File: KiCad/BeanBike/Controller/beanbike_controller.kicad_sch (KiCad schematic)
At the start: 1 part, among them U1 ESP32-WROOM-32

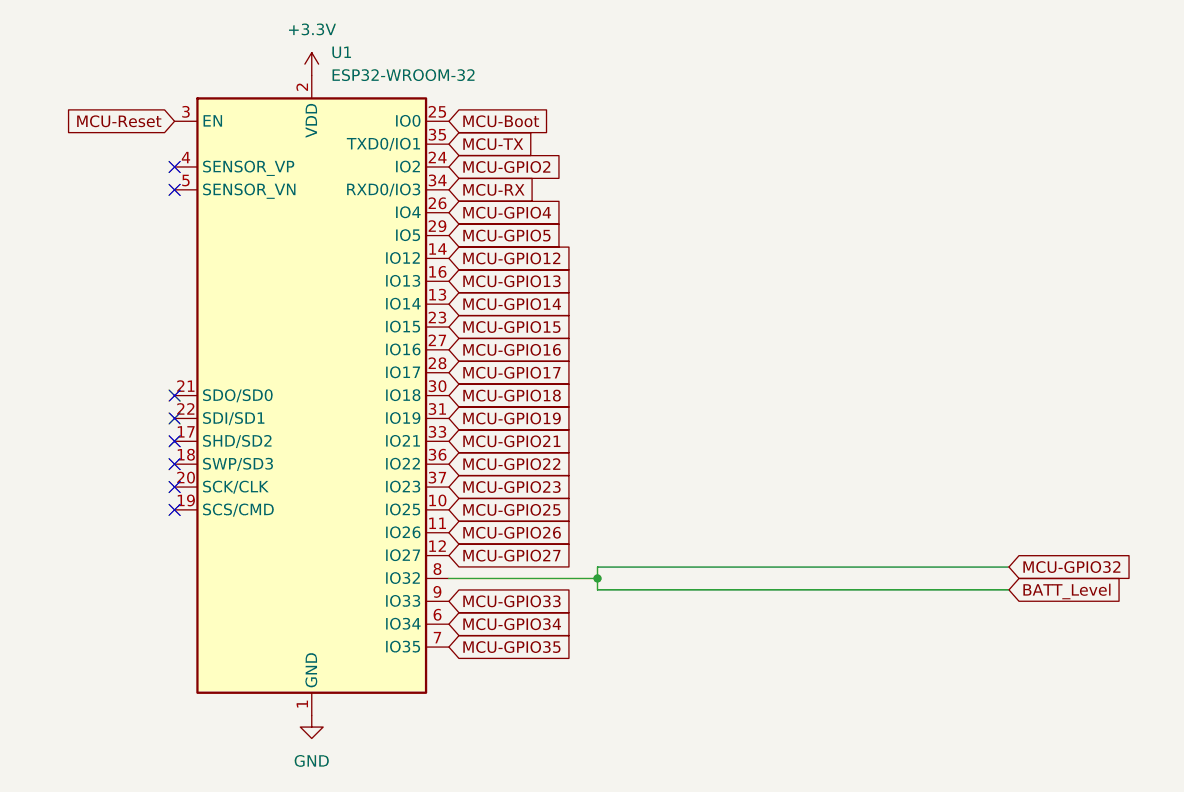
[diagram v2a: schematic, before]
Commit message: PCBv2 Finish
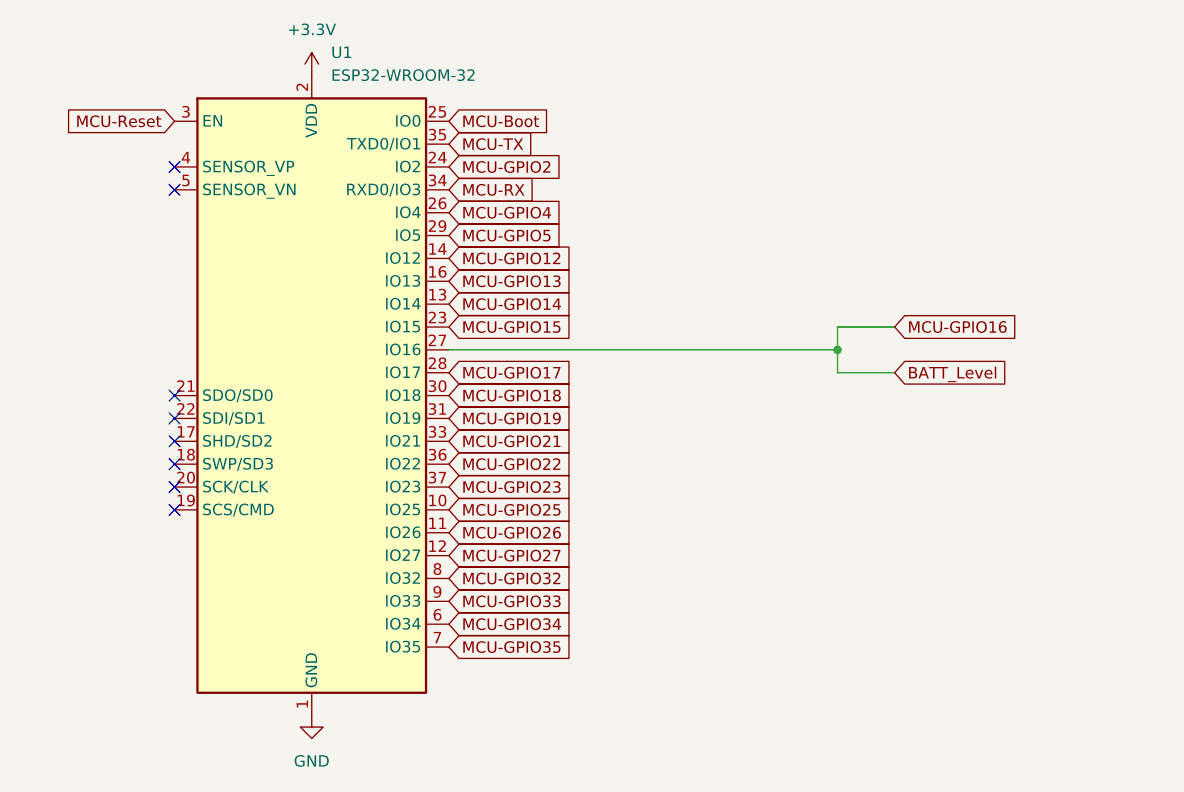
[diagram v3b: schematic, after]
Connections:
- net MCU-GPIO16 is gone; now on net BATT_Level: U1.27 (IO16)
- net BATT_Level: no longer U1.8 (IO32)
- new net MCU-GPIO32: U1.8 (IO32)
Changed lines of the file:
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@@
 	)
 	(junction
-		(at 167.64 130.81)
+		(at 194.31 105.41)
 		(diameter 0)
 		(color 0 0 0 0)
@@
 	(wire
 		(pts
-			(xy 213.36 129.54) (xy 167.64 129.54)
+			(xy 200.66 107.95) (xy 194.31 107.95)
 		)
 		(stroke
@@
 	(wire
 		(pts
-			(xy 167.64 130.81) (xy 167.64 132.08)
+			(xy 194.31 102.87) (xy 194.31 105.41)
 		)
 		(stroke
@@
 	(wire
 		(pts
-			(xy 167.64 130.81) (xy 151.13 130.81)
+			(xy 194.31 107.95) (xy 194.31 105.41)
 		)
 		(stroke
@@
 	(wire
 		(pts
-			(xy 167.64 129.54) (xy 167.64 130.81)
+			(xy 194.31 105.41) (xy 151.13 105.41)
 		)
 		(stroke
@@
 	(wire
 		(pts
-			(xy 167.64 132.08) (xy 213.36 132.08)
+			(xy 200.66 102.87) (xy 194.31 102.87)
 		)
 		(stroke
@@
 	(global_label "BATT_Level"
 		(shape input)
-		(at 213.36 132.08 0)
-		(fields_autoplaced yes)
-		(effects
-			(font
-				(size 1.27 1.27)
-			)
-			(justify left)
-		)
-		(property "Intersheetrefs" "${INTERSHEET_REFS}"
-			(at 226.4447 132.08 0)
+		(at 200.66 107.95 0)
+		(fields_autoplaced yes)
+		(effects
+			(font
+				(size 1.27 1.27)
+			)
+			(justify left)
+		)
+		(property "Intersheetrefs" "${INTERSHEET_REFS}"
+			(at 213.7447 107.95 0)
 			(effects
 				(font
@@
 	(global_label "MCU-GPIO32"
 		(shape input)
-		(at 213.36 129.54 0)
-		(fields_autoplaced yes)
-		(effects
-			(font
-				(size 1.27 1.27)
-			)
-			(justify left)
-		)
-		(property "Intersheetrefs" "${INTERSHEET_REFS}"
-			(at 228.8638 129.54 0)
+		(at 151.13 130.81 0)
+		(fields_autoplaced yes)
+		(effects
+			(font
+				(size 1.27 1.27)
+			)
+			(justify left)
+		)
+		(property "Intersheetrefs" "${INTERSHEET_REFS}"
+			(at 166.6338 130.81 0)
 			(effects
 				(font
@@
 	(global_label "MCU-GPIO16"
 		(shape input)
-		(at 151.13 105.41 0)
-		(fields_autoplaced yes)
-		(effects
-			(font
-				(size 1.27 1.27)
-			)
-			(justify left)
-		)
-		(property "Intersheetrefs" "${INTERSHEET_REFS}"
-			(at 166.6338 105.41 0)
-			(effects
-				(font
+		(at 200.66 102.87 0)
+		(fields_autoplaced yes)
+		(effects
+			(font
+				(size 1.27 1.27)
+			)
+			(justify left)
+		)
+		(property "Intersheetrefs" "${INTERSHEET_REFS}"
+			(at 216.1638 102.87 0)
+			(effects
+				(font

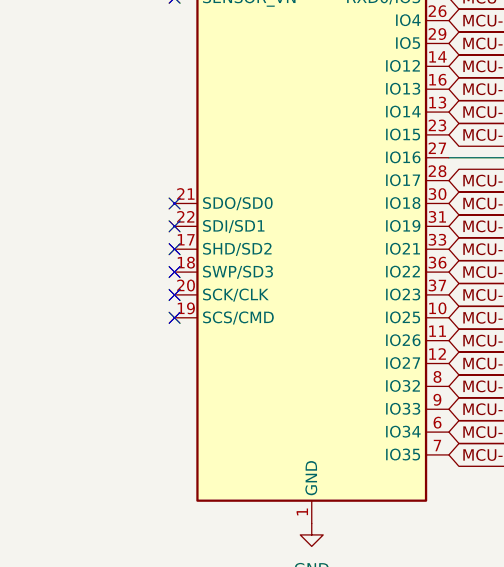
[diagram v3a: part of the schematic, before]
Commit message: More Firmware
😄
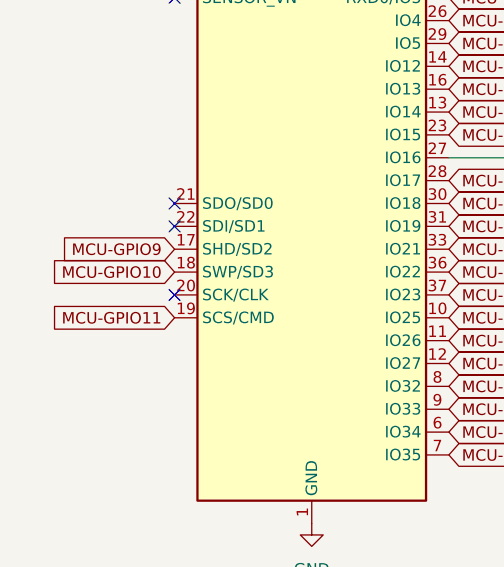
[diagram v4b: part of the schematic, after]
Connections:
- net MCU-GPIO9: now reaches U1.17 (SHD/SD2)
- net MCU-GPIO10: now reaches U1.18 (SWP/SD3)
- net MCU-GPIO11: now reaches U1.19 (SCS/CMD)
- no-connect marks 8 -> 5
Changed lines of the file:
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@@
-	)
-	(no_connect
-		(at 120.65 115.57)
 	)
 	(no_connect
@@
 	)
 	(no_connect
-		(at 120.65 123.19)
-	)
-	(no_connect
 		(at 120.65 87.63)
 	)
 	(no_connect
 		(at 120.65 85.09)
-	)
-	(no_connect
-		(at 120.65 118.11)
 	)
 	(wire
@@
 		)
 	)
+	(global_label "MCU-GPIO11"
+		(shape input)
+		(at 120.65 123.19 180)
+		(fields_autoplaced yes)
+		(effects
+			(font
+				(size 1.27 1.27)
+			)
+			(justify right)
+		)
+		(property "Intersheetrefs" "${INTERSHEET_REFS}"
+			(at 105.1462 123.19 0)
+			(effects
+				(font
+					(size 1.27 1.27)
+				)
+				(justify right)
+				(hide yes)
+			)
+		)
+	)
 	(global_label "MCU-GPIO19"
 		(shape input)
@@
 		)
 	)
+	(global_label "MCU-GPIO10"
+		(shape input)
+		(at 120.65 118.11 180)
+		(fields_autoplaced yes)
+		(effects
+			(font
+				(size 1.27 1.27)
+			)
+			(justify right)
+		)
+		(property "Intersheetrefs" "${INTERSHEET_REFS}"
+			(at 105.1462 118.11 0)
+			(effects
+				(font
+					(size 1.27 1.27)
+				)
+				(justify right)
+				(hide yes)
+			)
+		)
+	)
 	(global_label "MCU-GPIO4"
 		(shape input)
@@
 				(hide yes)
 			)
+		)
+	)
+	(global_label "MCU-GPIO9"
+		(shape input)
+		(at 120.65 115.57 180)
+		(fields_autoplaced yes)
+		(effects
+			(font
+				(size 1.27 1.27)
+			)
+			(justify right)
+		)
+		(property "Intersheetrefs" "${INTERSHEET_REFS}"
+			(at 106.3557 115.57 0)
+			(effects
+				(font
+					(size 1.27 1.27)
+				)
+				(justify right)
+				(hide yes)
+			)
